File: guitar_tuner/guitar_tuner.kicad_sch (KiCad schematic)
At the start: 8 parts, among them SW1 Reset, SW2 Boot, U1 ESP32-S2-SOLO

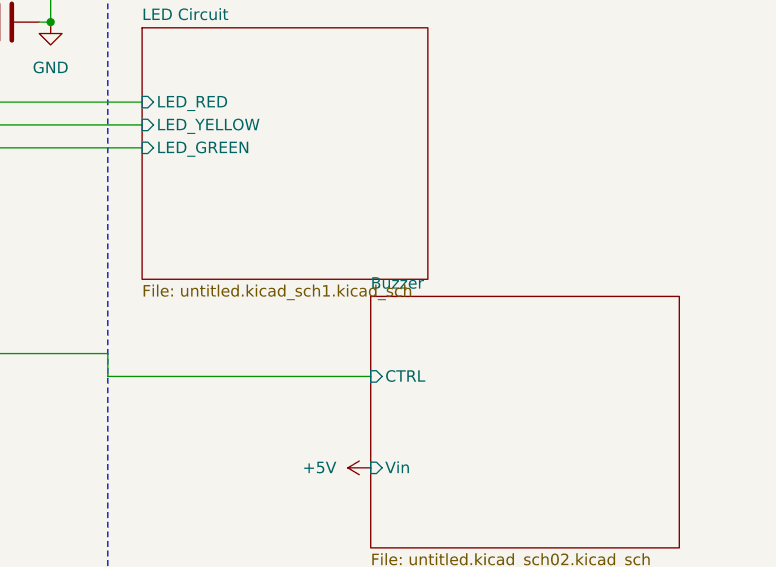
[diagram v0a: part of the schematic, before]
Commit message: Revert name change
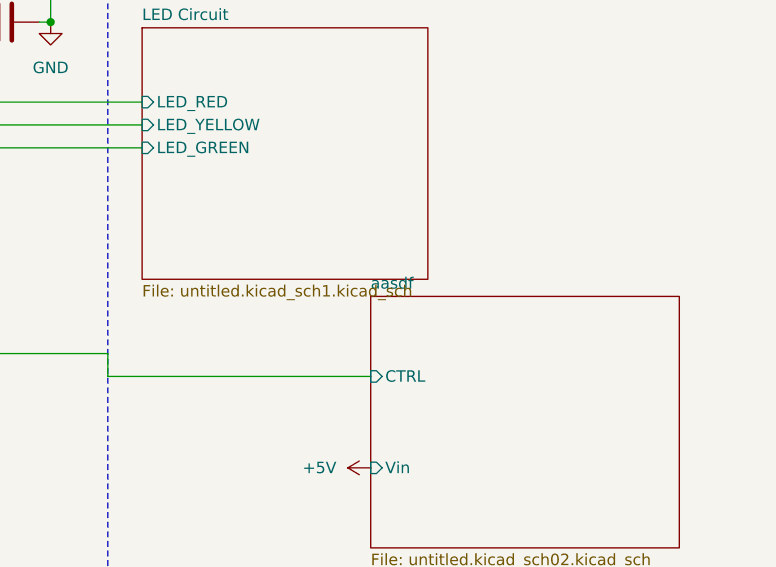
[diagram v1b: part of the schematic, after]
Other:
- sheet Buzzer renamed aasdf
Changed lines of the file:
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@@
 			(color 0 0 0 0.0000)
 		)
-		(property "Sheetname" "Buzzer"
+		(property "Sheetname" "aasdf"
 			(at 248.92 103.4284 0)
 			(effects
